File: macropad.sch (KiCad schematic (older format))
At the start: 13 parts

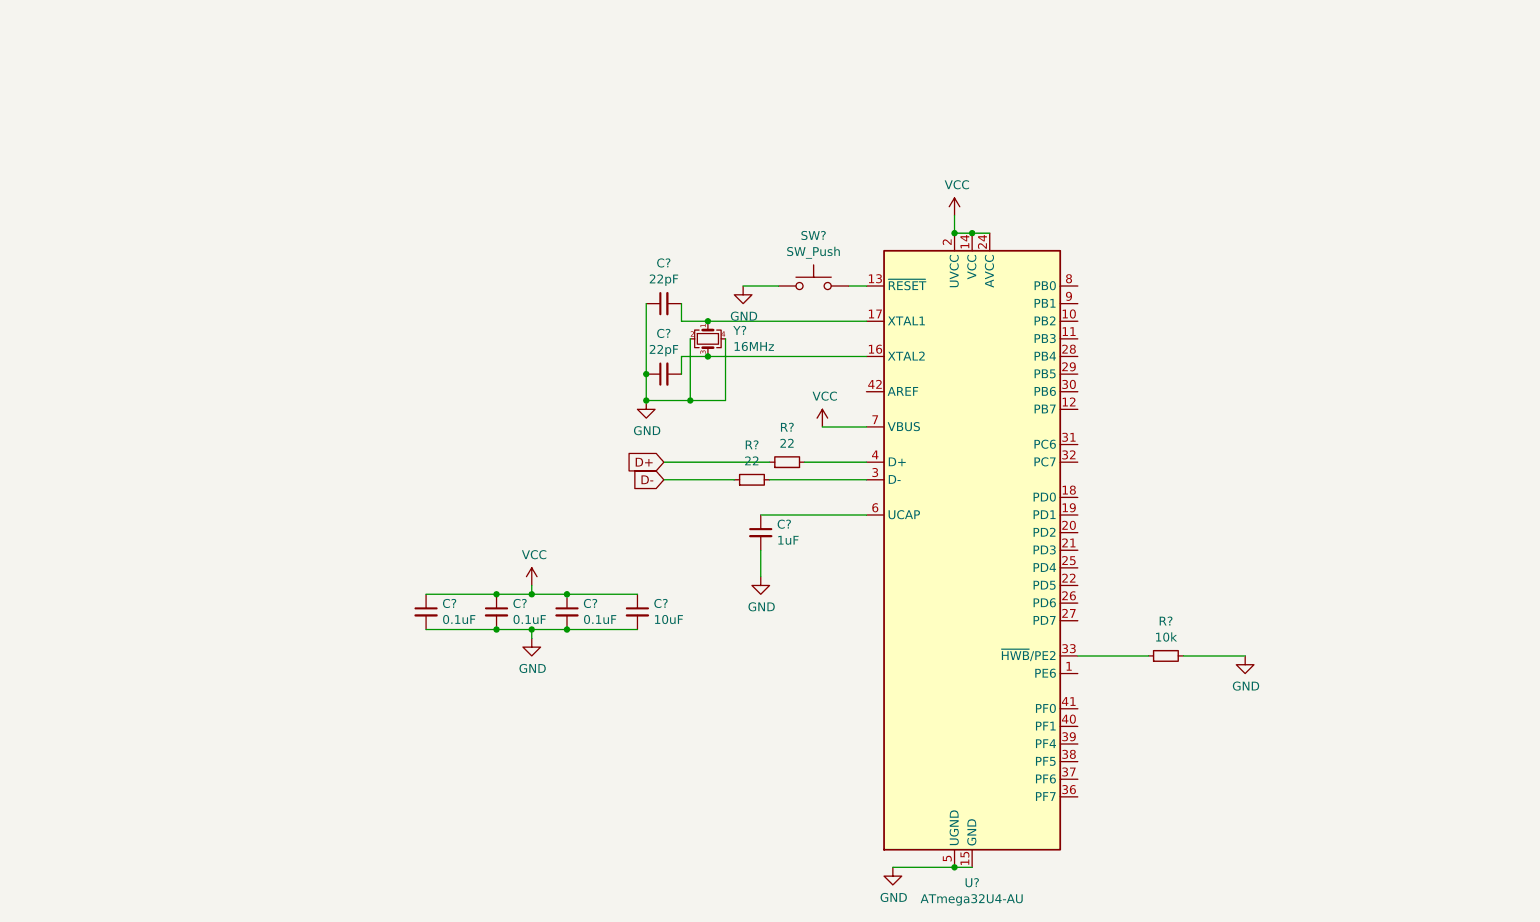
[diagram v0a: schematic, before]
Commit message: Power done, I think
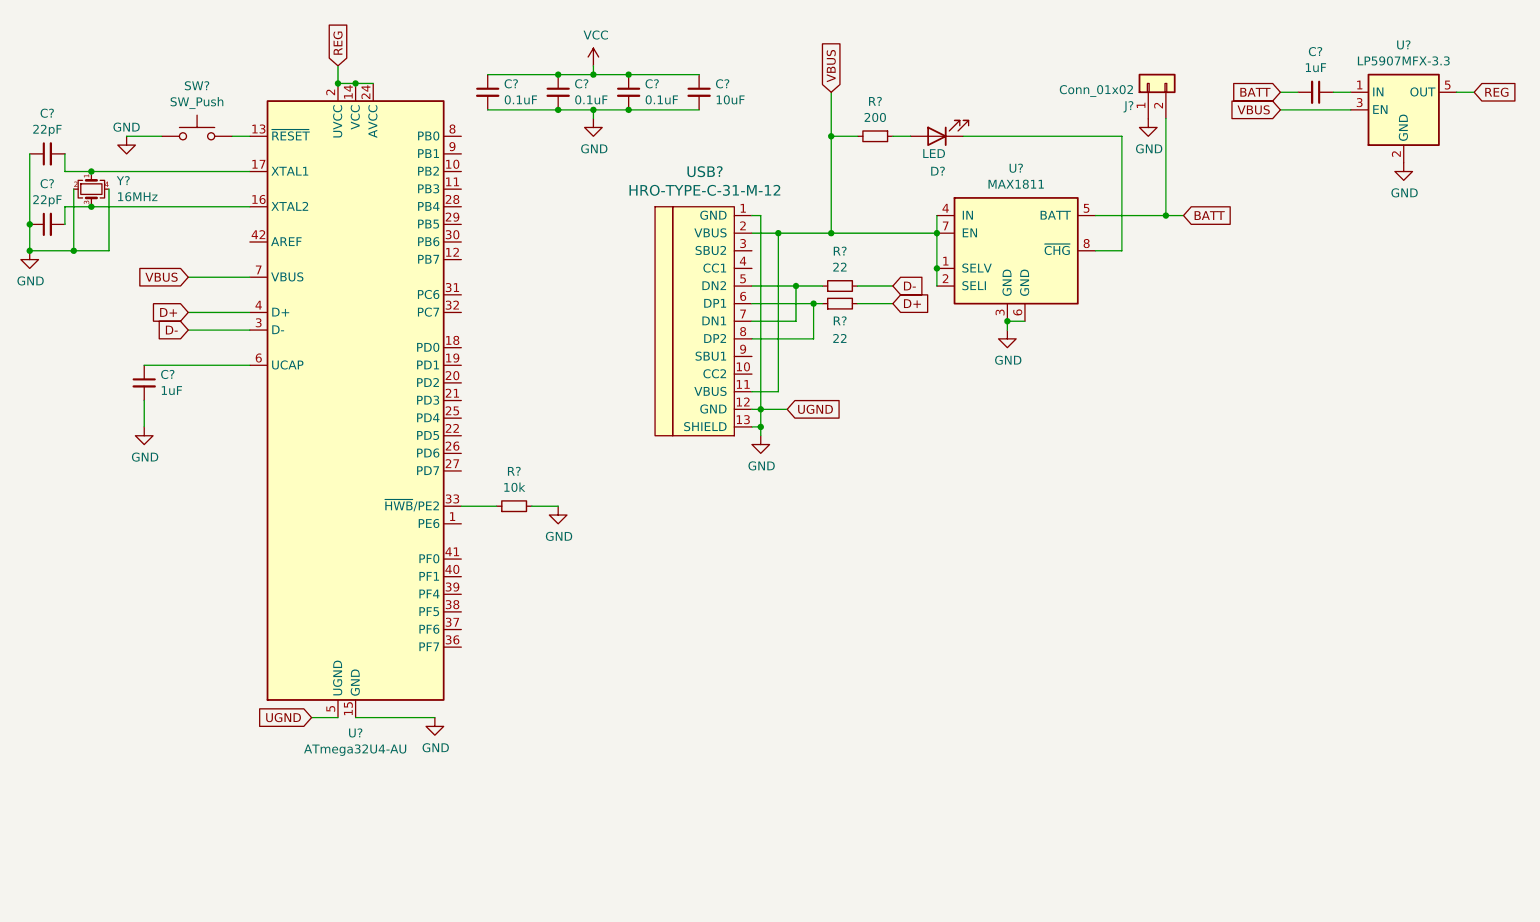
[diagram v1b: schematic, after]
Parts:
- added C?: 1uF, symbol Device:C_Small
- added D?: LED, symbol Device:LED
- added J?: Conn_01x02, symbol Connector_Generic:Conn_01x02
- added R?: 200, symbol Device:R_Small
- added U?: MAX1811, Package_SO:SOIC-8_3.9x4.9mm_P1.27mm, symbol Battery_Management:MAX1811
- added U?: LP5907MFX-3.3, Package_TO_SOT_SMD:SOT-23-5, symbol Regulator_Linear:LP5907MFX-3.3
- added USB?: HRO-TYPE-C-31-M-12, symbol Type-C:HRO-TYPE-C-31-M-12
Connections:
- net D+: now also R?.2, U?.4 (D+); no longer R?.1
- net D-: now also R?.2, U?.3 (D-); no longer R?.1
- net GND: now also J?.1 (Pin_1), U?.2 (GND), U?.3 (GND), U?.6 (GND), USB?.1 (GND), USB?.12 (GND), USB?.13 (SHIELD)
- net VCC: no longer U?.14 (VCC), U?.2 (UVCC), U?.24 (AVCC), U?.34 (VCC), U?.44 (AVCC), U?.7 (VBUS)
- new net: R?.1, USB?.5 (DN2), USB?.7 (DN1)
- new net: R?.1, USB?.6 (DP1), USB?.8 (DP2)
- new net: D?.1 (K), U?.8 (~CHG)
- new net: D?.2 (A), R?.1
- new net: C?.1, U?.1 (IN)
- new net BATT: C?.2, J?.2 (Pin_2), U?.5 (BATT)
- new net REG: U?.14 (VCC), U?.2 (UVCC), U?.24 (AVCC), U?.34 (VCC), U?.44 (AVCC), U?.5 (OUT)
- new net VBUS: R?.2, U?.1 (SELV), U?.2 (SELI), U?.3 (EN), U?.4 (IN), U?.7 (EN), U?.7 (VBUS), USB?.11 (VBUS), USB?.2 (VBUS)
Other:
- moved on the sheet: C?, R?, SW?, U?, Y?
